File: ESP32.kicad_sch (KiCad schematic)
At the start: 6 parts, among them U1 ESP32-C6-MINI-1

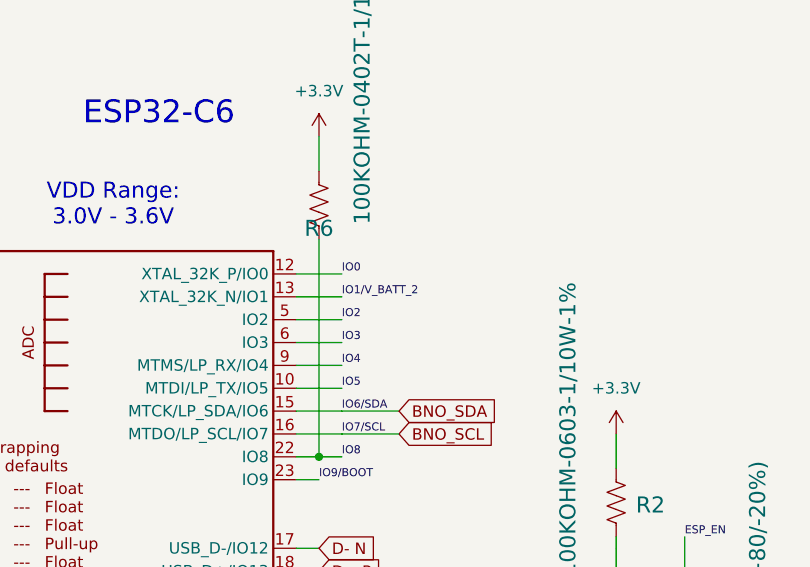
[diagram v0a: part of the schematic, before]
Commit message: PCB Smol Time
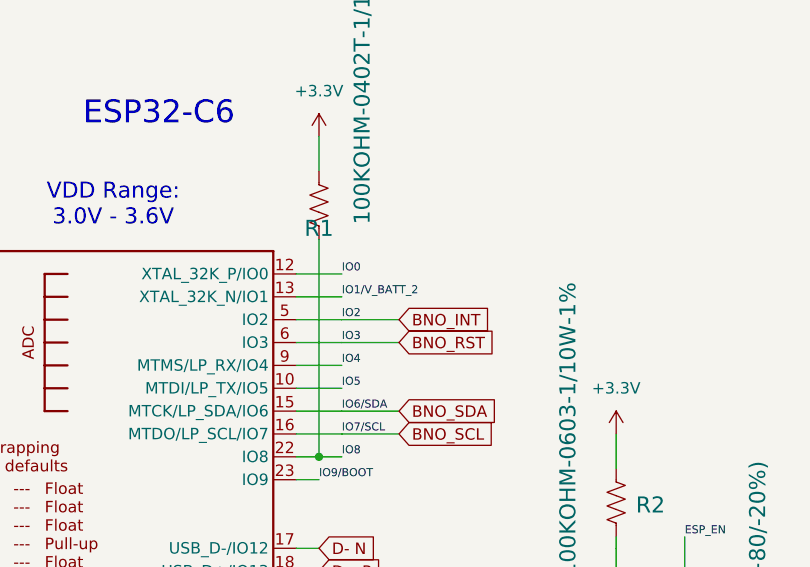
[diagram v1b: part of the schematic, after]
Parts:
- renumbered R6 to R1
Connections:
- net IO2 renamed BNO_INT
- net IO3 renamed BNO_RST
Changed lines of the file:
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@@
 	(wire
 		(pts
-			(xy 135.89 99.06) (xy 138.43 99.06)
-		)
-		(stroke
-			(width 0.1524)
-			(type solid)
-		)
-	)
-	(wire
-		(pts
-			(xy 135.89 91.44) (xy 140.97 91.44)
-		)
-		(stroke
-			(width 0.1524)
-			(type solid)
-		)
-	)
-	(wire
-		(pts
-			(xy 198.12 127) (xy 198.12 124.46)
-		)
-		(stroke
-			(width 0.1524)
-			(type solid)
-		)
-	)
-	(wire
-		(pts
-			(xy 138.43 114.3) (xy 135.89 114.3)
+			(xy 140.97 83.82) (xy 147.32 83.82)
 		)
 		(stroke
@@
 	(wire
 		(pts
+			(xy 135.89 99.06) (xy 138.43 99.06)
+		)
+		(stroke
+			(width 0.1524)
+			(type solid)
+		)
+	)
+	(wire
+		(pts
+			(xy 135.89 91.44) (xy 140.97 91.44)
+		)
+		(stroke
+			(width 0.1524)
+			(type solid)
+		)
+	)
+	(wire
+		(pts
+			(xy 198.12 127) (xy 198.12 124.46)
+		)
+		(stroke
+			(width 0.1524)
+			(type solid)
+		)
+	)
+	(wire
+		(pts
+			(xy 138.43 114.3) (xy 135.89 114.3)
+		)
+		(stroke
+			(width 0)
+			(type default)
+		)
+	)
+	(wire
+		(pts
 			(xy 135.89 83.82) (xy 140.97 83.82)
 		)
@@
 			(width 0.1524)
 			(type solid)
+		)
+	)
+	(wire
+		(pts
+			(xy 140.97 86.36) (xy 147.32 86.36)
+		)
+		(stroke
+			(width 0)
+			(type default)
 		)
 	)
@@
 		)
 	)
+	(global_label "BNO_INT"
+		(shape input)
+		(at 147.32 83.82 0)
+		(fields_autoplaced yes)
+		(effects
+			(font
+				(size 1.27 1.27)
+			)
+			(justify left)
+		)
+		(property "Intersheetrefs" "${INTERSHEET_REFS}"
+			(at 158.1067 83.82 0)
+			(effects
+				(font
+					(size 1.27 1.27)
+				)
+				(justify left)
+				(hide yes)
+			)
+		)
+	)
 	(global_label "D+ P"
 		(shape input)
@@
 		(property "Intersheetrefs" "${INTERSHEET_REFS}"
 			(at 146.5557 109.22 0)
+			(effects
+				(font
+					(size 1.27 1.27)
+				)
+				(justify left)
+				(hide yes)
+			)
+		)
+	)
+	(global_label "BNO_RST"
+		(shape input)
+		(at 147.32 86.36 0)
+		(fields_autoplaced yes)
+		(effects
+			(font
+				(size 1.27 1.27)
+			)
+			(justify left)
+		)
+		(property "Intersheetrefs" "${INTERSHEET_REFS}"
+			(at 158.6509 86.36 0)
 			(effects
 				(font
@@
 		(on_board yes)
 		(dnp no)
-		(property "Reference" "R6"
+		(property "Reference" "R1"
 			(at 138.43 72.644 0)
 			(effects
@@
 			(project "uSlime"
 				(path "/f32c1c49-f803-4e7c-a530-6db148a7ba36/27e9da7b-3bfa-4574-a980-93f02fcd8fa2"
-					(reference "R6")
+					(reference "R1")
 					(unit 1)
 				)
